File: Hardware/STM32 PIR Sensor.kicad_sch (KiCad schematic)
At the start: 28 parts

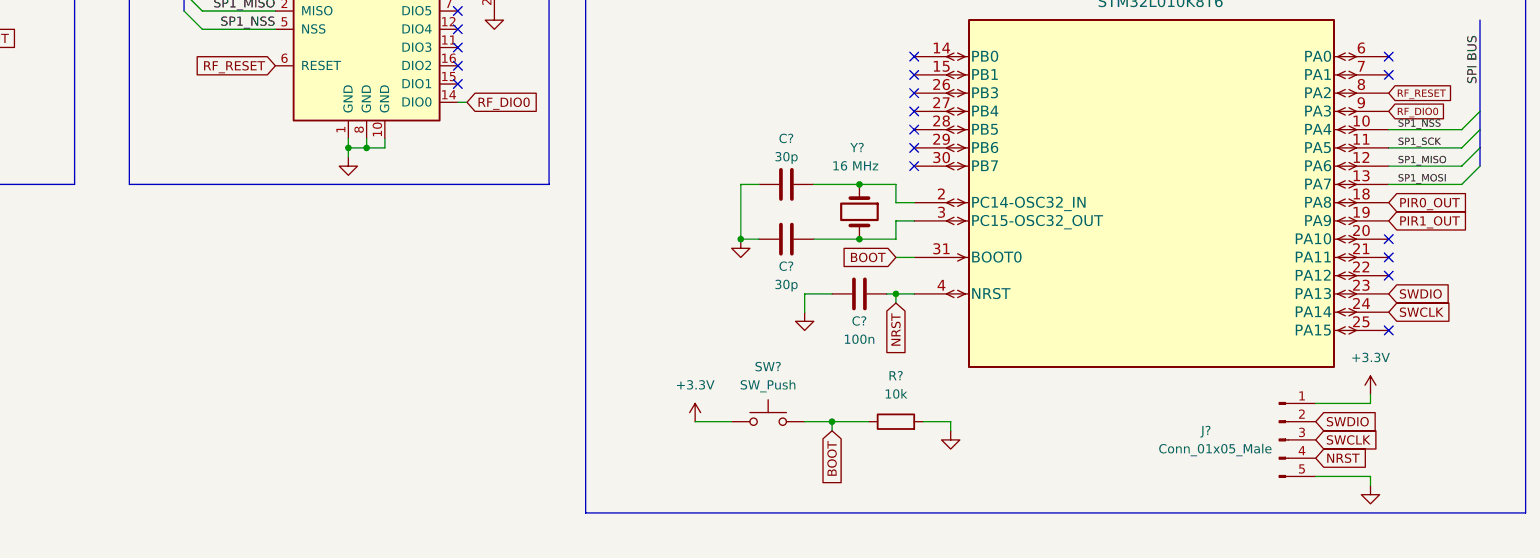
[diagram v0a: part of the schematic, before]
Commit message: v0.1 Schematic
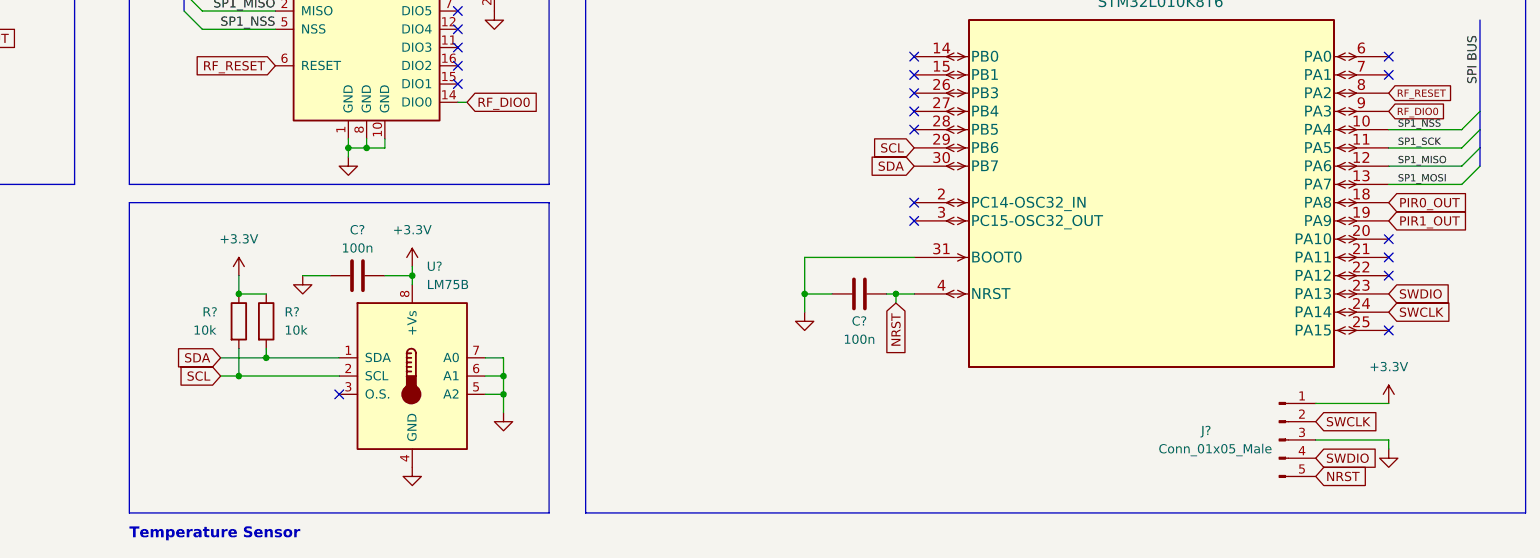
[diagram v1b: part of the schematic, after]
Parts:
- removed C? (x2): 30p, symbol Device:C
- removed R?: 10k, symbol Device:R
- removed SW?: SW_Push, symbol Switch:SW_Push
- removed Y?: 16 MHz, symbol Device:Crystal
- added C?: 100n, symbol Device:C
- added R? (x2): 10k, symbol Device:R
- added U?: LM75B, symbol Sensor_Temperature:LM75B
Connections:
- net BOOT is gone; now on net +3.3V: U?.31 (BOOT0)
- net +3.3V: now also J?.3 (Pin_3), C?.1, C?.2, R?.1, R?.1, U?.4 (GND), U?.5 (A2), U?.6 (A1), U?.7 (A0), U?.8 (+Vs); no longer J?.5 (Pin_5)
- net NRST: now also J?.5 (Pin_5); no longer J?.4 (Pin_4)
- net SWCLK: now also J?.2 (Pin_2); no longer J?.3 (Pin_3)
- net SWDIO: now also J?.4 (Pin_4); no longer J?.2 (Pin_2)
- net SCL: now reaches U?.29 (PB6)
- net SCL: now also R?.2, U?.2 (SCL)
- net SDA: now reaches U?.30 (PB7)
- net SDA: now also R?.2, U?.1 (SDA)
- no-connect marks 18 -> 19
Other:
- note added: "Temperature Sensor"
